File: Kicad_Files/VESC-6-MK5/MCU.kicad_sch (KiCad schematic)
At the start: 13 parts, among them U1 STM32F405RGTx, Y1 8M

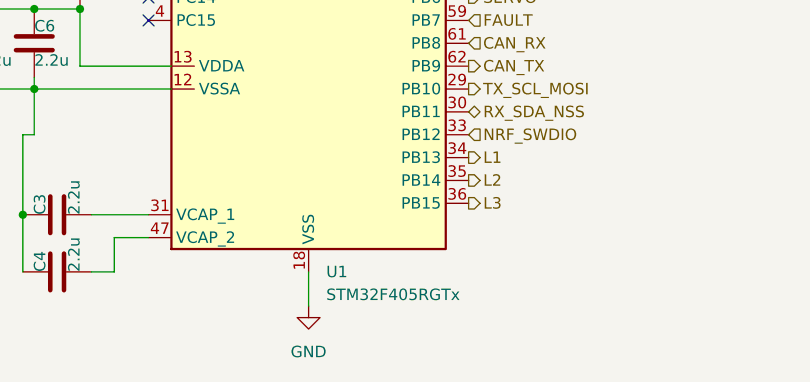
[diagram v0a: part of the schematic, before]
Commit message: Working sample of the display
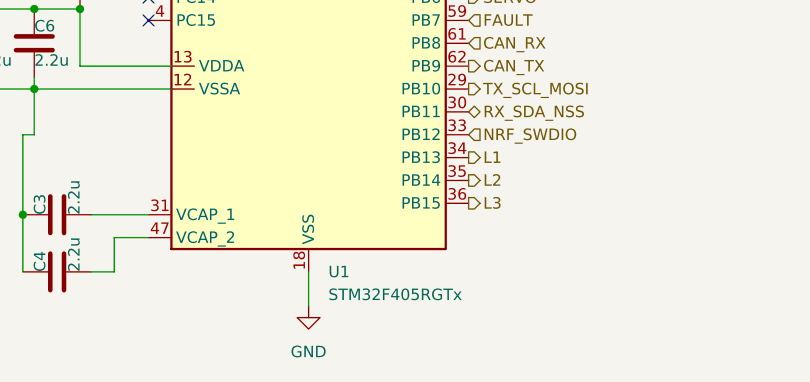
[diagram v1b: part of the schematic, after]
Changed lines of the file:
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@@
   (symbol (lib_id "MCU_ST_STM32F4:STM32F405RGTx") (at 140.97 88.9 0) (unit 1)
     (in_bom yes) (on_board yes) (dnp no) (fields_autoplaced)
-    (property "Reference" "U1" (at 142.9259 134.62 0)
-      (effects (font (size 1.27 1.27)) (justify left))
-    )
-    (property "Value" "STM32F405RGTx" (at 142.9259 137.16 0)
+    (property "Reference" "U1" (at 143.1641 134.62 0)
+      (effects (font (size 1.27 1.27)) (justify left))
+    )
+    (property "Value" "STM32F405RGTx" (at 143.1641 137.16 0)
       (effects (font (size 1.27 1.27)) (justify left))
     )
@@
       (effects (font (size 1.27 1.27)) hide)
     )
-    (property "Datasheet" "https://mm.digikey.com/Volume0/opasdata/d220001/medias/docus/503/CL05A104KA5NNNC.pdf" (at 109.22 48.26 0)
-      (effects (font (size 1.27 1.27)) hide)
-    )
+    (property "Datasheet" "CL05A104KA5NNNC" (at 109.22 48.26 0)
+      (effects (font (size 1.27 1.27)) hide)
+    )
